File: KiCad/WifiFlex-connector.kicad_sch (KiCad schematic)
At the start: 2 parts, among them J1 Conn_01x20_Pin, J2 Conn_01x06_Pin

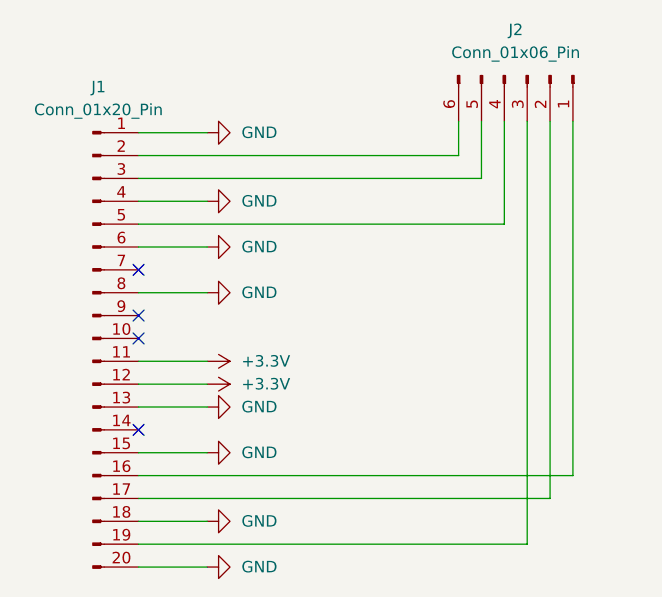
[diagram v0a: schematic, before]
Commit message: add modified files
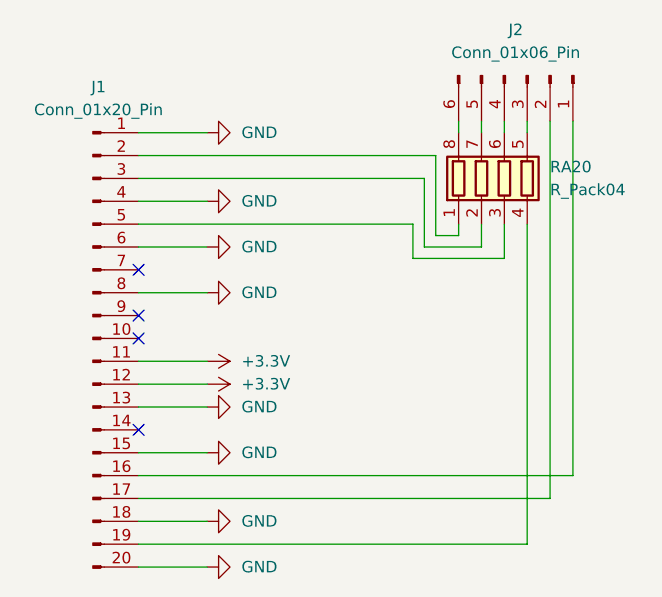
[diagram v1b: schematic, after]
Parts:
- added RA20: R_Pack04, Resistor_SMD:R_Array_Convex_4x0402, symbol Device:R_Pack04
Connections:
- net at J1.19 (Pin_19): now also RA20.4 (R4.1); no longer J2.3 (Pin_3)
- net at J1.5 (Pin_5): now also RA20.3 (R3.1); no longer J2.4 (Pin_4)
- net at J1.3 (Pin_3): now also RA20.2 (R2.1); no longer J2.5 (Pin_5)
- net at J1.2 (Pin_2): now also RA20.1 (R1.1); no longer J2.6 (Pin_6)
- new net: J2.3 (Pin_3), RA20.5 (R4.2)
- new net: J2.4 (Pin_4), RA20.6 (R3.2)
- new net: J2.5 (Pin_5), RA20.7 (R2.2)
- new net: J2.6 (Pin_6), RA20.8 (R1.2)
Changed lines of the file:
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@@
 	(wire
 		(pts
-			(xy 99.06 63.5) (xy 134.62 63.5)
-		)
-		(stroke
-			(width 0)
-			(type default)
-		)
-	)
-	(wire
-		(pts
-			(xy 139.7 71.12) (xy 139.7 59.69)
+			(xy 134.62 72.39) (xy 134.62 71.12)
+		)
+		(stroke
+			(width 0)
+			(type default)
+		)
+	)
+	(wire
+		(pts
+			(xy 99.06 63.5) (xy 132.08 63.5)
 		)
 		(stroke
@@
 	(wire
 		(pts
-			(xy 134.62 59.69) (xy 134.62 63.5)
-		)
-		(stroke
-			(width 0)
-			(type default)
-		)
-	)
-	(wire
-		(pts
 			(xy 99.06 78.74) (xy 106.68 78.74)
 		)
@@
 	(wire
 		(pts
+			(xy 99.06 71.12) (xy 129.54 71.12)
+		)
+		(stroke
+			(width 0)
+			(type default)
+		)
+	)
+	(wire
+		(pts
 			(xy 99.06 101.6) (xy 144.78 101.6)
 		)
@@
 	(wire
 		(pts
-			(xy 99.06 66.04) (xy 137.16 66.04)
-		)
-		(stroke
-			(width 0)
-			(type default)
-		)
-	)
-	(wire
-		(pts
-			(xy 142.24 106.68) (xy 142.24 59.69)
-		)
-		(stroke
-			(width 0)
-			(type default)
-		)
-	)
-	(wire
-		(pts
-			(xy 99.06 71.12) (xy 139.7 71.12)
+			(xy 134.62 60.96) (xy 134.62 59.69)
+		)
+		(stroke
+			(width 0)
+			(type default)
+		)
+	)
+	(wire
+		(pts
+			(xy 142.24 106.68) (xy 142.24 71.12)
+		)
+		(stroke
+			(width 0)
+			(type default)
+		)
+	)
+	(wire
+		(pts
+			(xy 132.08 72.39) (xy 134.62 72.39)
+		)
+		(stroke
+			(width 0)
+			(type default)
+		)
+	)
+	(wire
+		(pts
+			(xy 139.7 60.96) (xy 139.7 59.69)
+		)
+		(stroke
+			(width 0)
+			(type default)
+		)
+	)
+	(wire
+		(pts
+			(xy 130.81 66.04) (xy 130.81 73.66)
 		)
 		(stroke
@@
 	(wire
 		(pts
+			(xy 137.16 60.96) (xy 137.16 59.69)
+		)
+		(stroke
+			(width 0)
+			(type default)
+		)
+	)
+	(wire
+		(pts
 			(xy 144.78 101.6) (xy 144.78 59.69)
 		)
@@
 	(wire
 		(pts
-			(xy 137.16 66.04) (xy 137.16 59.69)
+			(xy 99.06 66.04) (xy 130.81 66.04)
+		)
+		(stroke
+			(width 0)
+			(type default)
+		)
+	)
+	(wire
+		(pts
+			(xy 132.08 63.5) (xy 132.08 72.39)
+		)
+		(stroke
+			(width 0)
+			(type default)
+		)
+	)
+	(wire
+		(pts
+			(xy 130.81 73.66) (xy 137.16 73.66)
+		)
+		(stroke
+			(width 0)
+			(type default)
+		)
+	)
+	(wire
+		(pts
+			(xy 139.7 71.12) (xy 139.7 74.93)
+		)
+		(stroke
+			(width 0)
+			(type default)
+		)
+	)
+	(wire
+		(pts
+			(xy 142.24 60.96) (xy 142.24 59.69)
+		)
+		(stroke
+			(width 0)
+			(type default)
+		)
+	)
+	(wire
+		(pts
+			(xy 129.54 74.93) (xy 139.7 74.93)
+		)
+		(stroke
+			(width 0)
+			(type default)
+		)
+	)
+	(wire
+		(pts
+			(xy 129.54 71.12) (xy 129.54 74.93)
 		)
 		(stroke
@@
 		(pts
 			(xy 99.06 91.44) (xy 106.68 91.44)
+		)
+		(stroke
+			(width 0)
+			(type default)
+		)
+	)
+	(wire
+		(pts
+			(xy 137.16 71.12) (xy 137.16 73.66)
 		)
 		(stroke
@@
 					(unit 1)
 				)
+			)
+		)
+	)
+	(symbol
+		(lib_id "Device:R_Pack04")
+		(at 139.7 66.04 0)
+		(unit 1)
+		(exclude_from_sim no)
+		(in_bom yes)
+		(on_board yes)
+		(dnp no)
+		(fields_autoplaced yes)
+		(property "Reference" "RA20"
+			(at 144.78 64.7699 0)
+			(effects
+				(font
+					(size 1.27 1.27)
+				)
+				(justify left)
+			)
+		)
+		(property "Value" "R_Pack04"
+			(at 144.78 67.3099 0)
+			(effects
+				(font
+					(size 1.27 1.27)
+				)
+				(justify left)
+			)
+		)
+		(property "Footprint" "Resistor_SMD:R_Array_Convex_4x0402"
+			(at 146.685 66.04 90)
+			(effects
+				(font
+					(size 1.27 1.27)
+				)
+				(hide yes)
+			)
+		)
+		(property "Datasheet" "~"
+			(at 139.7 66.04 0)
+			(effects
+				(font
+					(size 1.27 1.27)
+				)
+				(hide yes)
+			)
+		)
+		(property "Description" "4 resistor network, parallel topology"
+			(at 139.7 66.04 0)
+			(effects
+				(font
+					(size 1.27 1.27)
+				)
+				(hide yes)
+			)
+		)
+		(pin "6"
+		)
+		(pin "2"
+		)
+		(pin "3"
+		)
+		(pin "1"
+		)
+		(pin "7"
+		)
+		(pin "4"
+		)
+		(pin "8"
+		)
+		(pin "5"
+		)
+		(instances
+			(project "WifiFlex-connector"
+				(path "/77b97498-b9b7-43e2-89cb-7947d298f0c2"
+					(reference "RA20")
+					(unit 1)
+				)
